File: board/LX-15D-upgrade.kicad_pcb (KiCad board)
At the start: 2 copper layers, 19 x 29 mm, 37 parts, among them J1 M+, J2 M-, J3 IN-1, J4 IN-2, J5 SWD, U1 DRV8801A-Q1, U2 AS5600, U3 MPU-6050, U4 STM32L011F4Px, U5 AP7383-W5-3V3

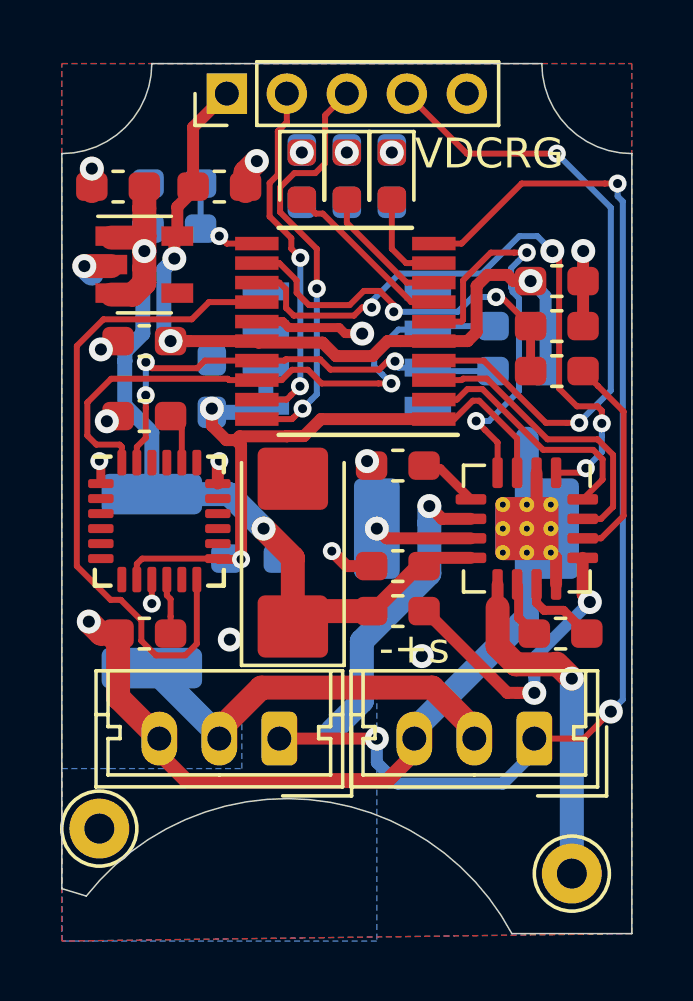
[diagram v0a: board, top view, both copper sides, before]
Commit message: Final tweak
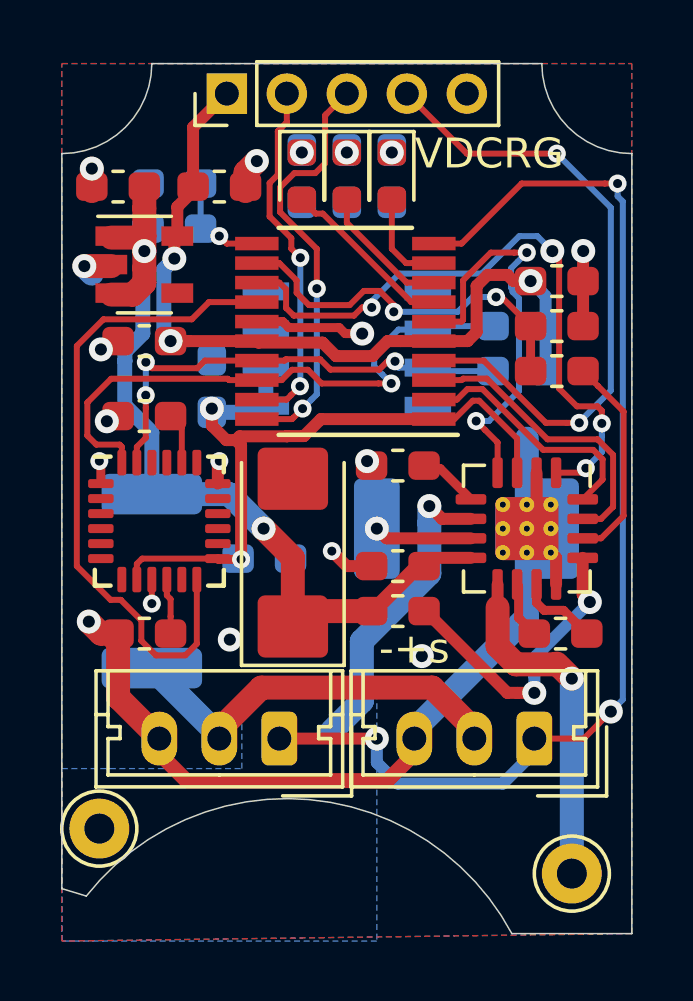
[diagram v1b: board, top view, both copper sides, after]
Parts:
- moved C6 0.38 mm to (147.2, 107.0)
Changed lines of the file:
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@@
   )
   (module Capacitor_SMD:C_0603_1608Metric_Pad1.05x0.95mm_HandSolder (layer B.Cu)
-    (at 146.875 107 180)
+    (at 147.25 107 180)
     (descr "Capacitor SMD 0603 (1608 Metric), square (rectangular) end terminal, IPC_7351 nominal with elongated pad for handsoldering. (Body size source: http://www.tortai-tech.com/upload/download/2011102023233369053.pdf), generated with kicad-footprint-generator")
     (tags "capacitor handsolder")
